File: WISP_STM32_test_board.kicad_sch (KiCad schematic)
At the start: 43 parts, among them J1 Conn_02x05_Odd_Even, J4 Conn_01x10_Pin, J5 Conn_01x02_Pin, J6 Conn_01x03_Socket, J7 Conn_01x03_Socket, SW1 SW_Push, SW2 SW_Push, SW5 SW_SPST, U1 MAX3072E, U2 MAX3072E, U4 STM32F446RETx, U6 AP63203WU

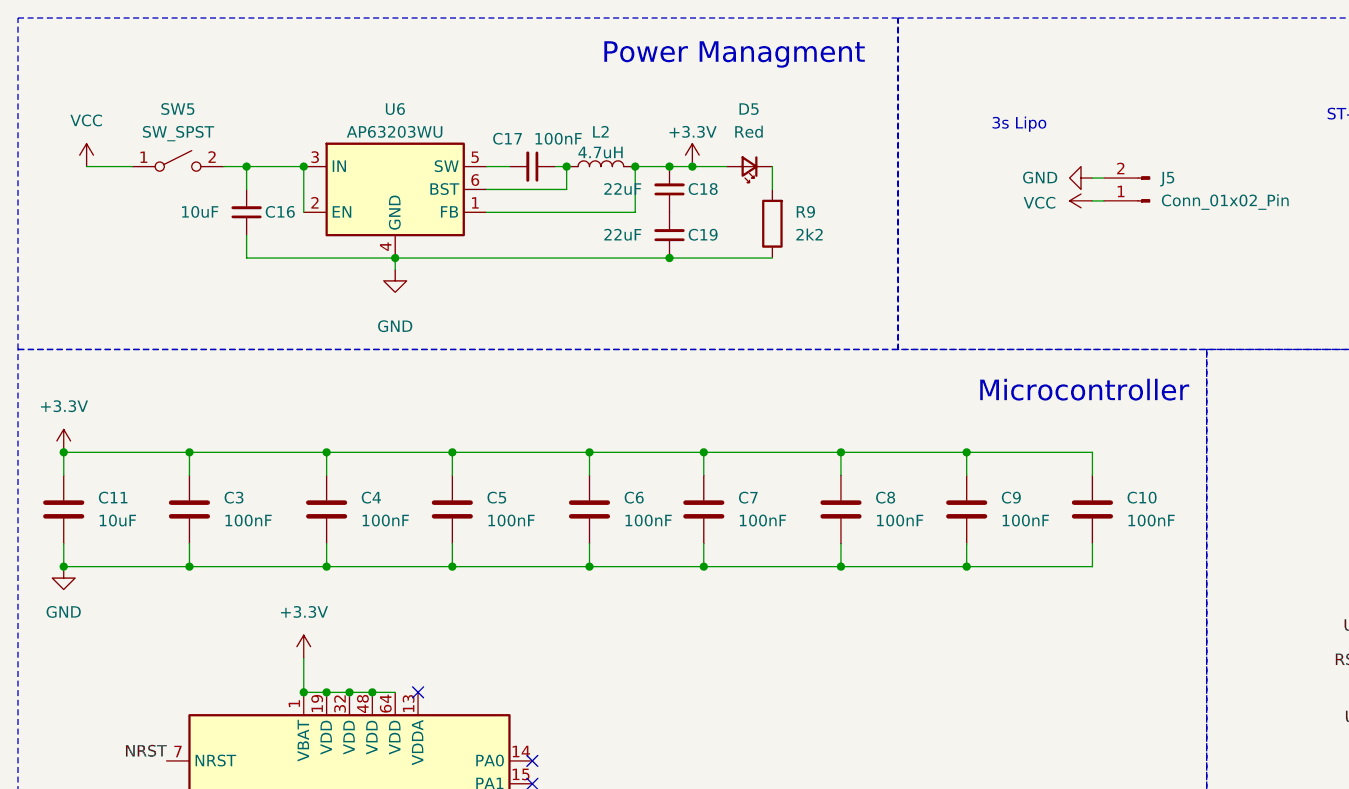
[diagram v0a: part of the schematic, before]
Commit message: Rough draft V4
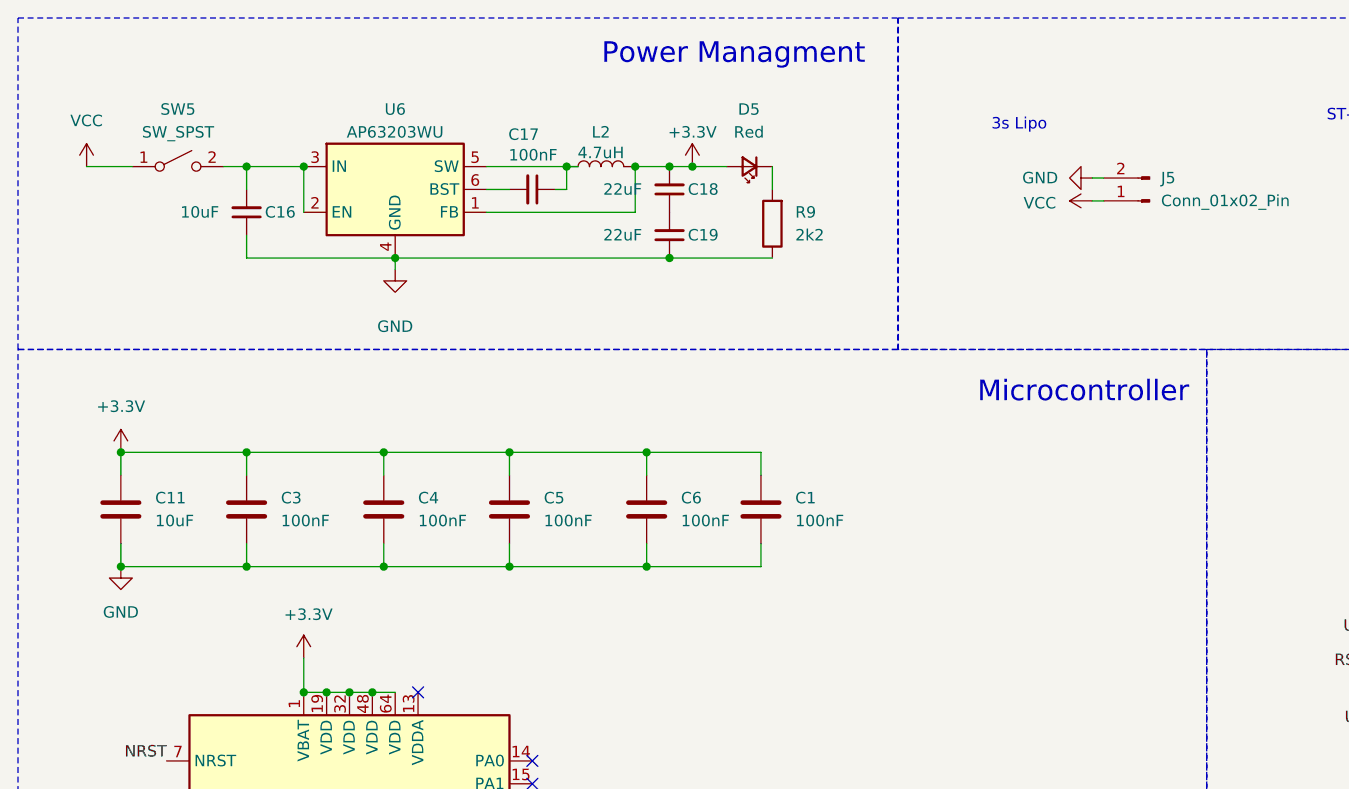
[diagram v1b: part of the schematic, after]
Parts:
- removed C10, C7, C8, C9: 100nF, Capacitor_SMD:C_0805_2012Metric_Pad1.18x1.45mm_HandSolder, symbol Device:C
- added C1: 100nF, Capacitor_SMD:C_0603_1608Metric, symbol Device:C
- C11, C3, C4, C5, C6: footprint Capacitor_SMD:C_0805_2012Metric_Pad1.18x1.45mm_HandSolder -> Capacitor_SMD:C_0603_1608Metric
- L2: footprint Inductor_SMD:L_0805_2012Metric_Pad1.05x1.20mm_HandSolder -> Inductor_SMD:L_Taiyo-Yuden_MD-4040
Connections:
- net +3.3V: now also C1.1
- net GND: now also C1.2
- net at U6.5 (SW): now also C17.1, L2.1; no longer C17.2
- new net: C17.2, U6.6 (BST)
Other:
- moved on the sheet: C11, C17, C3, C4, C5, C6
